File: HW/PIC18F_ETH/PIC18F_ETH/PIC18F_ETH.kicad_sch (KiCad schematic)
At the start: 0 parts

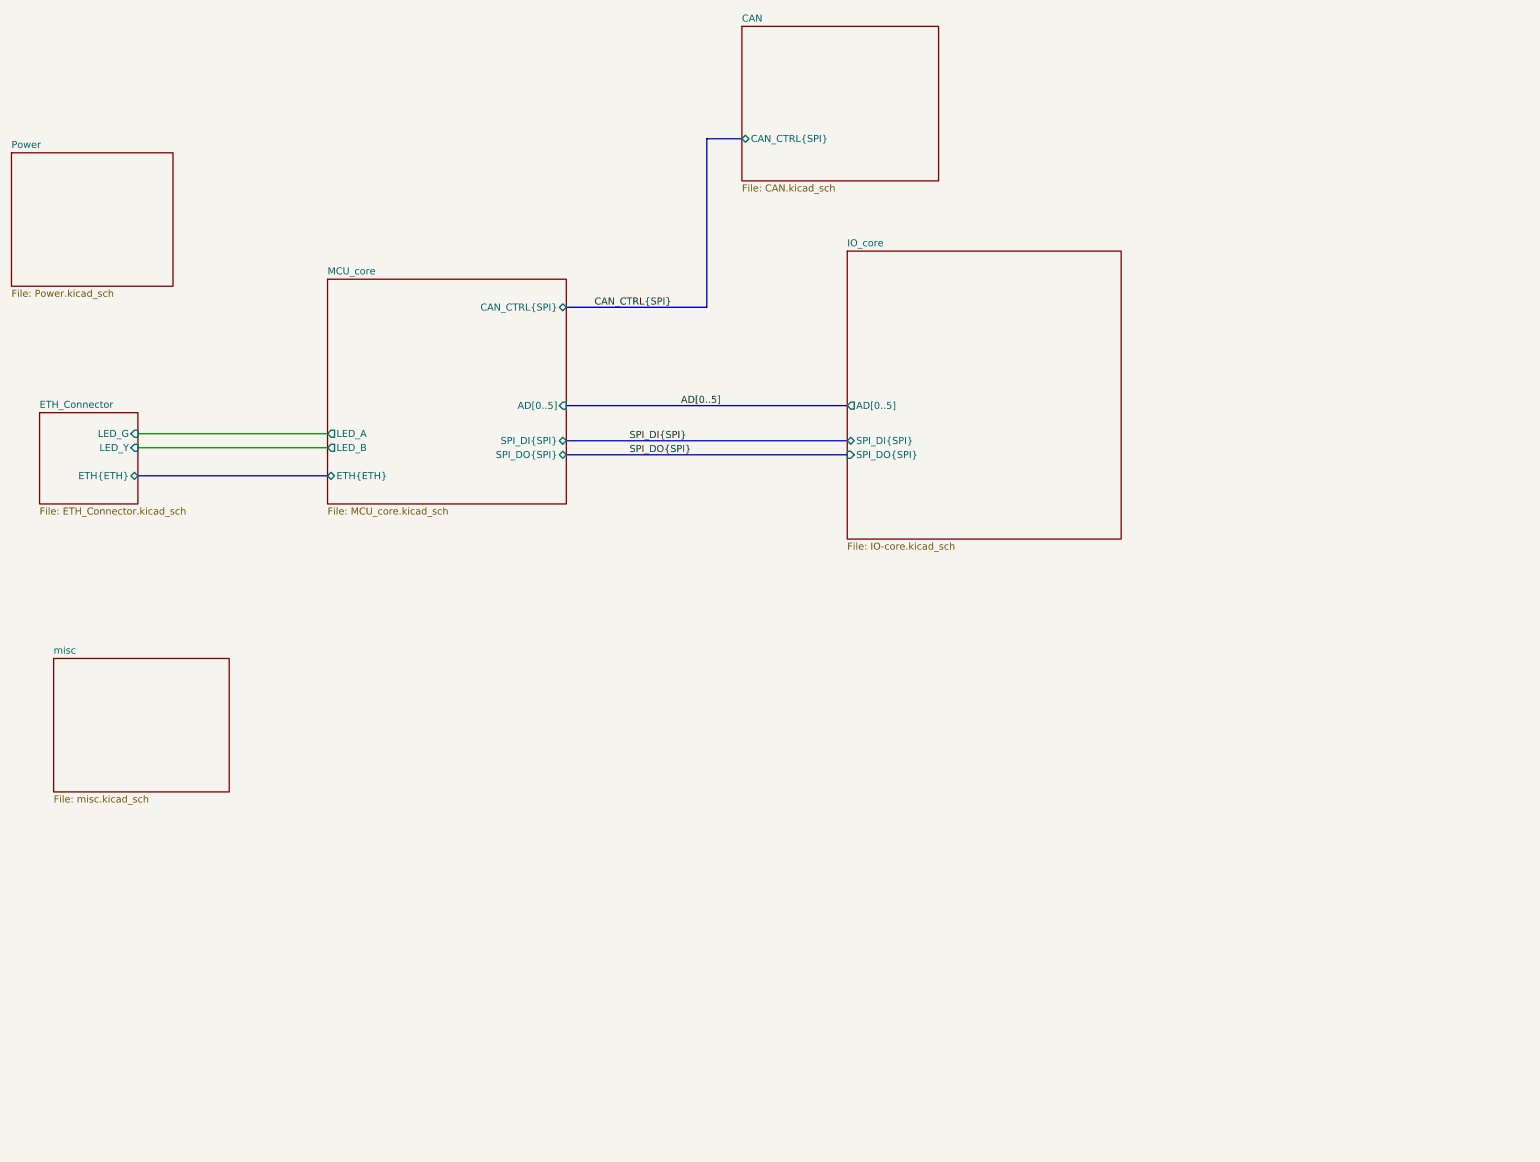
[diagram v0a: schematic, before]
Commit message: .
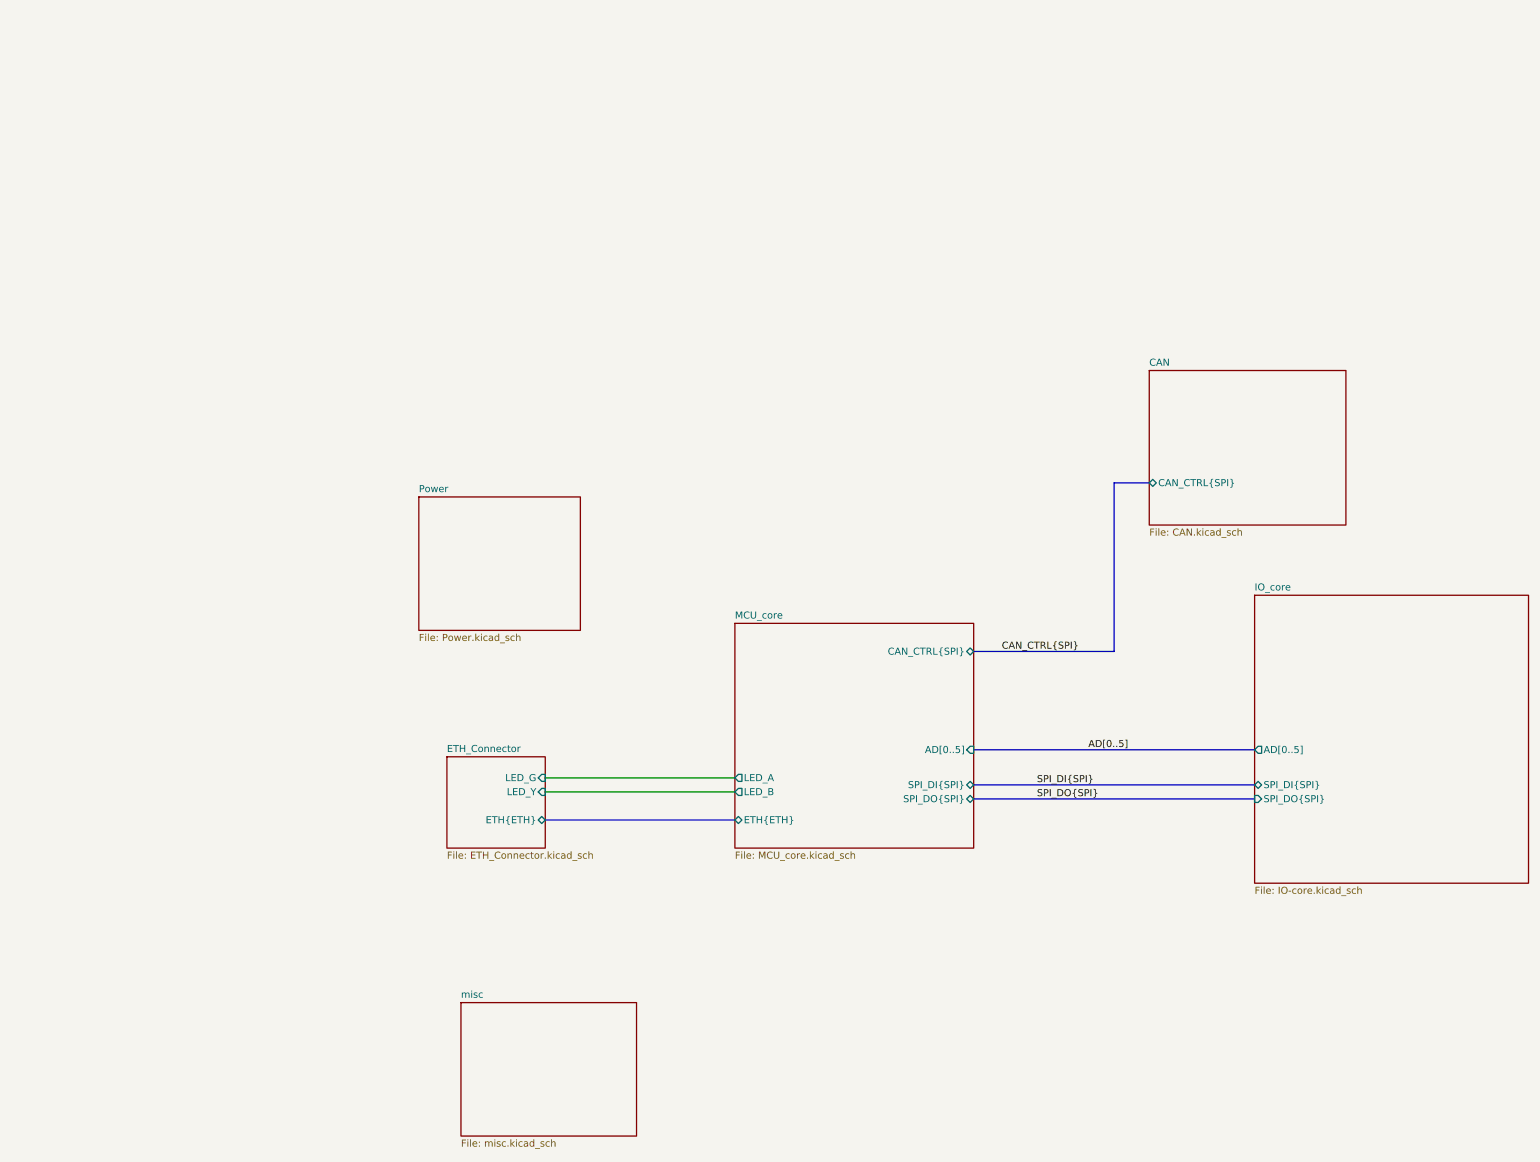
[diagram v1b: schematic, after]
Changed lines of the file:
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@@
 	(generator "eeschema")
 	(generator_version "8.0")
-	(paper "A4")
-	(bus
-		(pts
-			(xy 158.75 96.52) (xy 209.55 96.52)
-		)
-		(stroke
-			(width 0)
-			(type default)
-		)
-	)
-	(bus
-		(pts
-			(xy 158.75 105.41) (xy 209.55 105.41)
-		)
-		(stroke
-			(width 0)
-			(type default)
-		)
-	)
-	(bus
-		(pts
-			(xy 184.15 78.74) (xy 158.75 78.74)
-		)
-		(stroke
-			(width 0)
-			(type default)
-		)
-	)
-	(bus
-		(pts
-			(xy 184.15 48.26) (xy 184.15 78.74)
+	(paper "A3")
+	(bus
+		(pts
+			(xy 232.41 158.75) (xy 283.21 158.75)
+		)
+		(stroke
+			(width 0)
+			(type default)
+		)
+	)
+	(bus
+		(pts
+			(xy 232.41 167.64) (xy 283.21 167.64)
+		)
+		(stroke
+			(width 0)
+			(type default)
+		)
+	)
+	(bus
+		(pts
+			(xy 257.81 140.97) (xy 232.41 140.97)
+		)
+		(stroke
+			(width 0)
+			(type default)
+		)
+	)
+	(bus
+		(pts
+			(xy 257.81 110.49) (xy 257.81 140.97)
 		)
 		(stroke
@@
 	(wire
 		(pts
-			(xy 81.28 104.14) (xy 115.57 104.14)
+			(xy 154.94 166.37) (xy 189.23 166.37)
 		)
 		(stroke
@@
 	(wire
 		(pts
-			(xy 81.28 101.6) (xy 115.57 101.6)
-		)
-		(stroke
-			(width 0)
-			(type default)
-		)
-	)
-	(bus
-		(pts
-			(xy 158.75 102.87) (xy 209.55 102.87)
-		)
-		(stroke
-			(width 0)
-			(type default)
-		)
-	)
-	(bus
-		(pts
-			(xy 81.28 109.22) (xy 115.57 109.22)
-		)
-		(stroke
-			(width 0)
-			(type default)
-		)
-	)
-	(bus
-		(pts
-			(xy 190.5 48.26) (xy 184.15 48.26)
+			(xy 154.94 163.83) (xy 189.23 163.83)
+		)
+		(stroke
+			(width 0)
+			(type default)
+		)
+	)
+	(bus
+		(pts
+			(xy 232.41 165.1) (xy 283.21 165.1)
+		)
+		(stroke
+			(width 0)
+			(type default)
+		)
+	)
+	(bus
+		(pts
+			(xy 154.94 171.45) (xy 189.23 171.45)
+		)
+		(stroke
+			(width 0)
+			(type default)
+		)
+	)
+	(bus
+		(pts
+			(xy 264.16 110.49) (xy 257.81 110.49)
 		)
 		(stroke
@@
 	)
 	(label "SPI_DI{SPI}"
-		(at 170.18 102.87 0)
+		(at 243.84 165.1 0)
 		(fields_autoplaced yes)
 		(effects
@@
 	)
 	(label "CAN_CTRL{SPI}"
-		(at 163.83 78.74 0)
+		(at 237.49 140.97 0)
 		(fields_autoplaced yes)
 		(effects
@@
 	)
 	(label "SPI_DO{SPI}"
-		(at 170.18 105.41 0)
+		(at 243.84 167.64 0)
 		(fields_autoplaced yes)
 		(effects
@@
 	)
 	(label "AD[0..5]"
-		(at 186.69 96.52 180)
+		(at 260.35 158.75 180)
 		(fields_autoplaced yes)
 		(effects
@@
 	)
 	(sheet
-		(at 209.55 68.58)
+		(at 283.21 130.81)
 		(size 49.53 52.07)
 		(fields_autoplaced yes)
@@
 		)
 		(property "Sheetname" "IO_core"
-			(at 209.55 67.8684 0)
+			(at 283.21 130.0984 0)
 			(effects
 				(font
@@
 		)
 		(property "Sheetfile" "IO-core.kicad_sch"
-			(at 209.55 121.2346 0)
+			(at 283.21 183.4646 0)
 			(effects
 				(font
@@
 		)
 		(pin "AD[0..5]" output
-			(at 209.55 96.52 180)
+			(at 283.21 158.75 180)
 			(effects
 				(font
@@
 		)
 		(pin "SPI_DO{SPI}" input
-			(at 209.55 105.41 180)
+			(at 283.21 167.64 180)
 			(effects
 				(font
@@
 		)
 		(pin "SPI_DI{SPI}" bidirectional
-			(at 209.55 102.87 180)
+			(at 283.21 165.1 180)
 			(effects
 				(font
@@
 	)
 	(sheet
-		(at 66.04 142.24)
+		(at 139.7 204.47)
 		(size 31.75 24.13)
 		(fields_autoplaced yes)
@@
 		)
 		(property "Sheetname" "misc"
-			(at 66.04 141.5284 0)
+			(at 139.7 203.7584 0)
 			(effects
 				(font
@@
 		)
 		(property "Sheetfile" "misc.kicad_sch"
-			(at 66.04 166.9546 0)
+			(at 139.7 229.1846 0)
 			(effects
 				(font
@@
 	)
 	(sheet
-		(at 190.5 27.94)
+		(at 264.16 90.17)
 		(size 35.56 27.94)
 		(fields_autoplaced yes)
@@
 		)
 		(property "Sheetname" "CAN"
-			(at 190.5 27.2284 0)
+			(at 264.16 89.4584 0)
 			(effects
 				(font
@@
 		)
 		(property "Sheetfile" "CAN.kicad_sch"
-			(at 190.5 56.4646 0)
+			(at 264.16 118.6946 0)
 			(effects
 				(font
@@
 		)
 		(pin "CAN_CTRL{SPI}" bidirectional
-			(at 190.5 48.26 180)
+			(at 264.16 110.49 180)
 			(effects
 				(font
@@
 	)
 	(sheet
-		(at 115.57 73.66)
+		(at 189.23 135.89)
 		(size 43.18 40.64)
 		(fields_autoplaced yes)
@@
 		)
 		(property "Sheetname" "MCU_core"
-			(at 115.57 72.9484 0)
+			(at 189.23 135.1784 0)
 			(effects
 				(font
@@
 		)
 		(property "Sheetfile" "MCU_core.kicad_sch"
-			(at 115.57 114.8846 0)
+			(at 189.23 177.1146 0)
 			(effects
 				(font
@@
 		)
 		(pin "ETH{ETH}" bidirectional
-			(at 115.57 109.22 180)
+			(at 189.23 171.45 180)
 			(effects
 				(font
@@
 		)
 		(pin "LED_B" output
-			(at 115.57 104.14 180)
+			(at 189.23 166.37 180)
 			(effects
 				(font
@@
 		)
 		(pin "LED_A" output
-			(at 115.57 101.6 180)
+			(at 189.23 163.83 180)
 			(effects
 				(font
@@
 		)
 		(pin "AD[0..5]" input
-			(at 158.75 96.52 0)
+			(at 232.41 158.75 0)
 			(effects
 				(font
@@
 		)
 		(pin "CAN_CTRL{SPI}" bidirectional
-			(at 158.75 78.74 0)
+			(at 232.41 140.97 0)
 			(effects
 				(font
@@
 		)
 		(pin "SPI_DI{SPI}" bidirectional
-			(at 158.75 102.87 0)
+			(at 232.41 165.1 0)
 			(effects
 				(font
@@
 		)
 		(pin "SPI_DO{SPI}" bidirectional
-			(at 158.75 105.41 0)
+			(at 232.41 167.64 0)
 			(effects
 				(font
@@
 	)
 	(sheet
-		(at 58.42 50.8)
+		(at 132.08 113.03)
 		(size 29.21 24.13)
 		(fields_autoplaced yes)
@@
 		)
 		(property "Sheetname" "Power"
-			(at 58.42 50.0884 0)
+			(at 132.08 112.3184 0)
 			(effects
 				(font
@@
 		)
 		(property "Sheetfile" "Power.kicad_sch"
-			(at 58.42 75.5146 0)
+			(at 132.08 137.7446 0)
 			(effects
 				(font
@@
 	)
 	(sheet
-		(at 63.5 97.79)
+		(at 137.16 160.02)
 		(size 17.78 16.51)
 		(fields_autoplaced yes)
@@
 		)
 		(property "Sheetname" "ETH_Connector"
-			(at 63.5 97.0784 0)
+			(at 137.16 159.3084 0)
 			(effects
 				(font
@@
 		)
 		(property "Sheetfile" "ETH_Connector.kicad_sch"
-			(at 63.5 114.8846 0)
+			(at 137.16 177.1146 0)
 			(effects
 				(font
@@
 		)
 		(pin "LED_G" input
-			(at 81.28 101.6 0)
+			(at 154.94 163.83 0)
 			(effects
 				(font
@@
 		)
 		(pin "LED_Y" input
-			(at 81.28 104.14 0)
+			(at 154.94 166.37 0)
 			(effects
 				(font
@@
 		)
 		(pin "ETH{ETH}" bidirectional
-			(at 81.28 109.22 0)
-			(effects
-				(font
+			(at 154.94 171.45 0)
+			(effects
+				(font
